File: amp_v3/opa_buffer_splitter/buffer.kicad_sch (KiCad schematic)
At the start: 16 parts, among them J10 OP_PWR, J11 AUDIO_IN, J12 AUDIO_OUT, U3 OPA1656

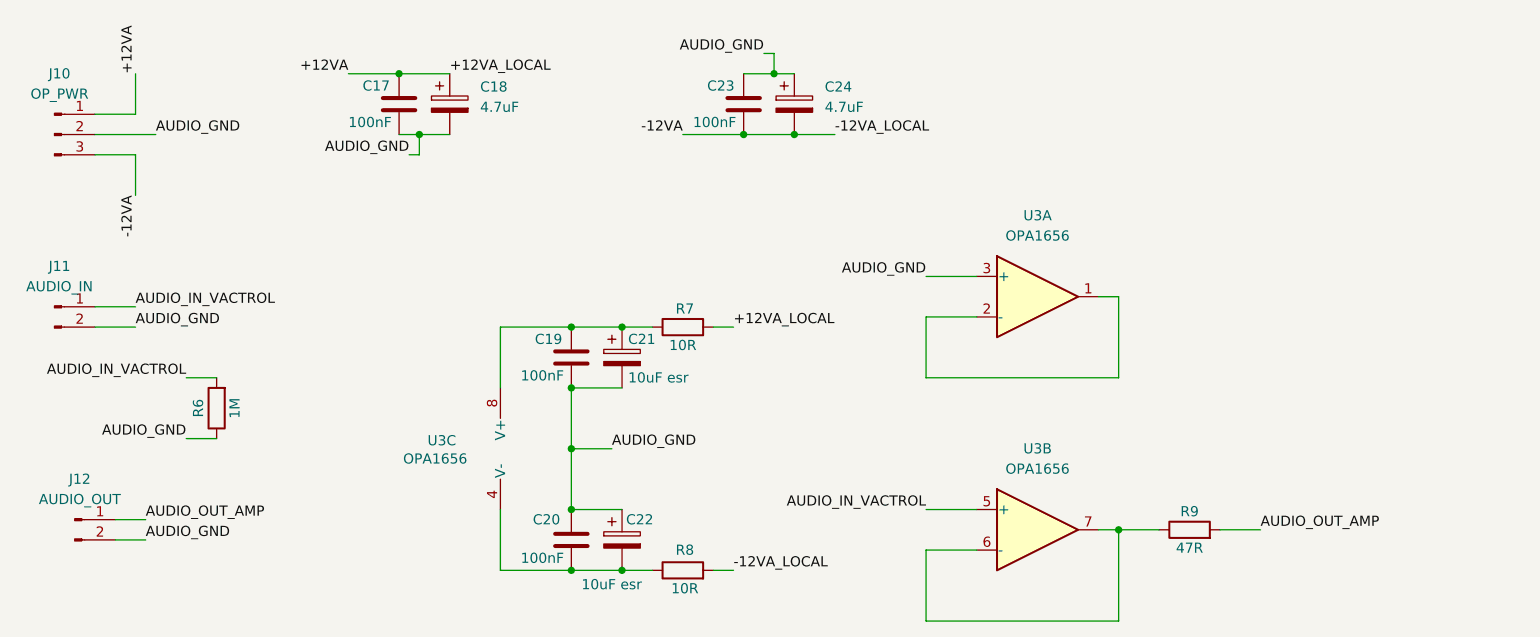
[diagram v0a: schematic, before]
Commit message: updates
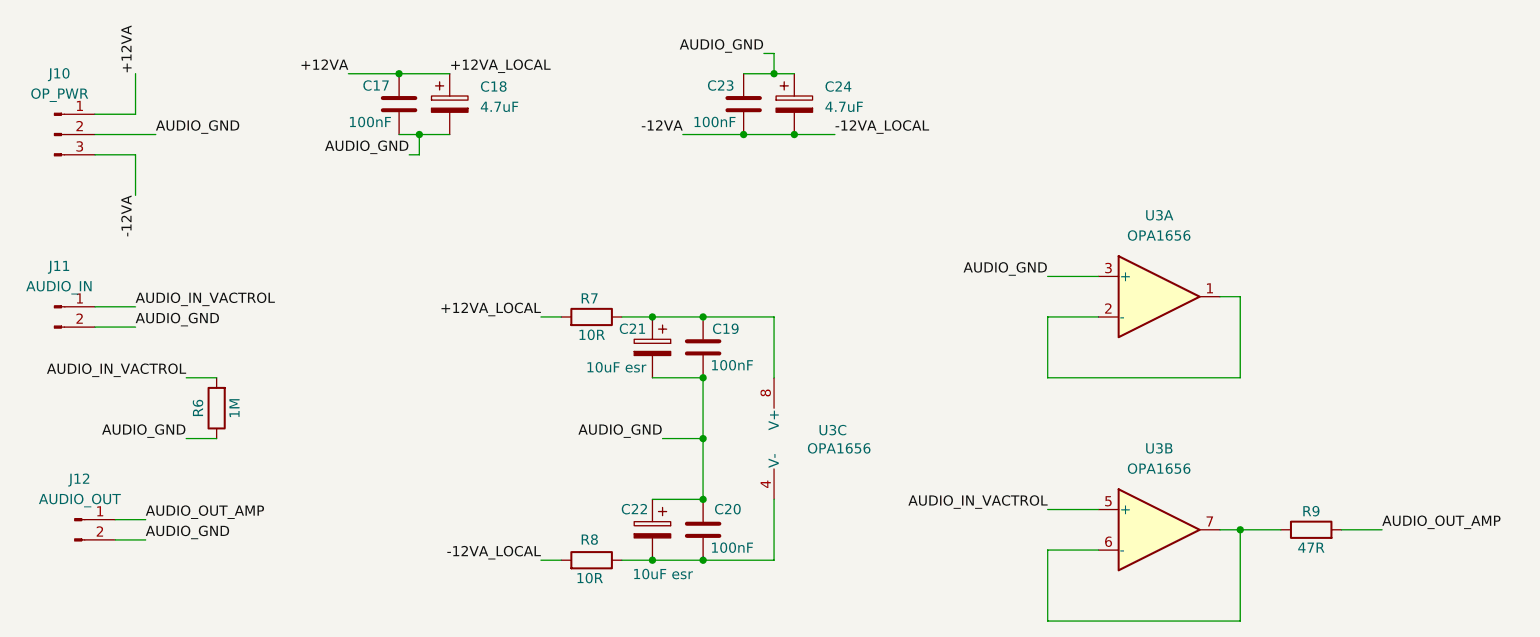
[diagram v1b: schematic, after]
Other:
- moved on the sheet: C19, C20, C21, C22, R7, R8, R9, U3A, U3B, U3C
